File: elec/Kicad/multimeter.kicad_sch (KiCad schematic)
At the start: 0 parts

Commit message: multimetring
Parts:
- added R18, R21: 9996, symbol Device:R
- added R22, R23: 833, symbol Device:R
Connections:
- new net: R18.2, R23.1
- new net: R21.2, R22.2
- new net GND: R22.1, R23.2
- new net read_pin_high: R21.1
- new net read_pin_low: R18.1
- no-connect marks 0 -> 2

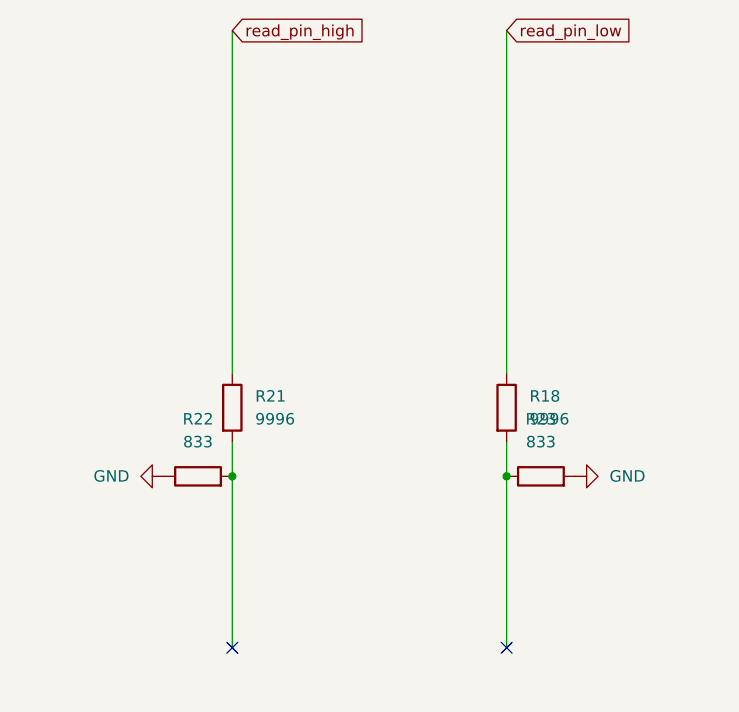
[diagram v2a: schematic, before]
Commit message: multimetrie
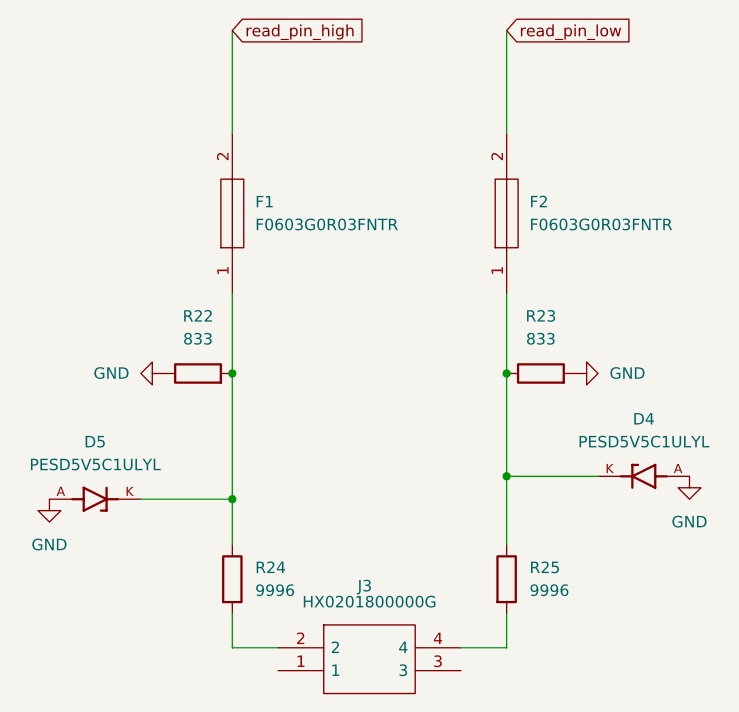
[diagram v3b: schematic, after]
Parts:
- removed R18, R21: 9996, symbol Device:R
- added D4, D5: PESD5V5C1ULYL, PESD5V5C1ULYL:DIO_PESD5V5C1ULYL, symbol PESD5V5C1ULYL:PESD5V5C1ULYL
- added F1, F2: F0603G0R03FNTR, F0603G0R03FNTR, symbol F0603G0R03FNTR:F0603G0R03FNTR
- added J3: HX0201800000G, HX0201800000G, symbol HX0201800000G:HX0201800000G
- added R24, R25: 9996, symbol Device:R
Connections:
- net GND: now also D4.A, D5.A
- net read_pin_high: now also F1.2
- net read_pin_low: now also F2.2
- net at R23.1: now also D4.K, F2.1, R25.1
- net at R22.2: now also D5.K, F1.1, R24.1
- new net: J3.2, R24.2
- new net: J3.4, R25.2
- no-connect marks 2 -> 0
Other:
- moved on the sheet: R22, R23
